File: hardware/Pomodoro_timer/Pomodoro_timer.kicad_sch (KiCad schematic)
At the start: 0 parts

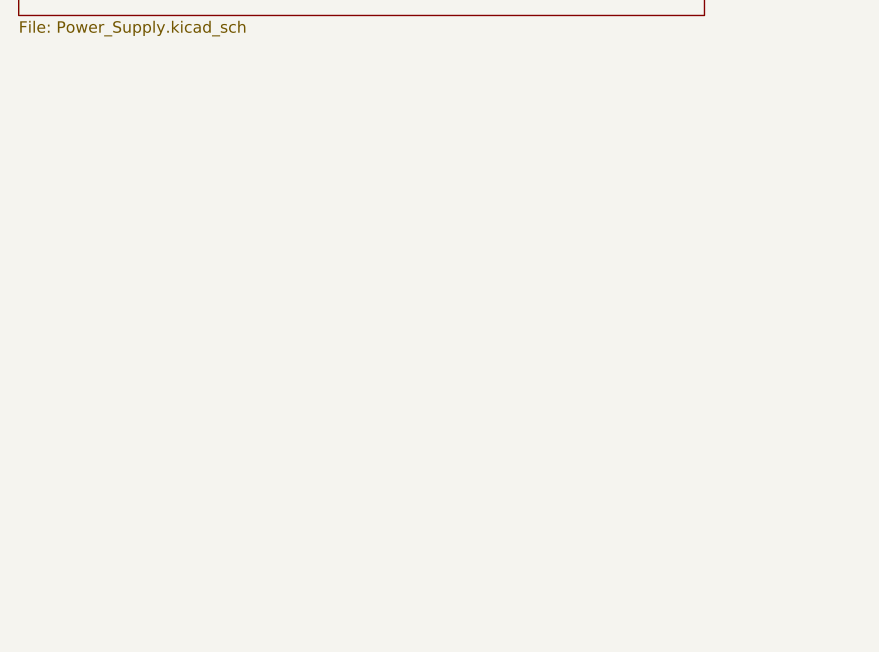
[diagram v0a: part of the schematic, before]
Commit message: PCB Ver.A : The Schematic completed the next part for PCB can be started.
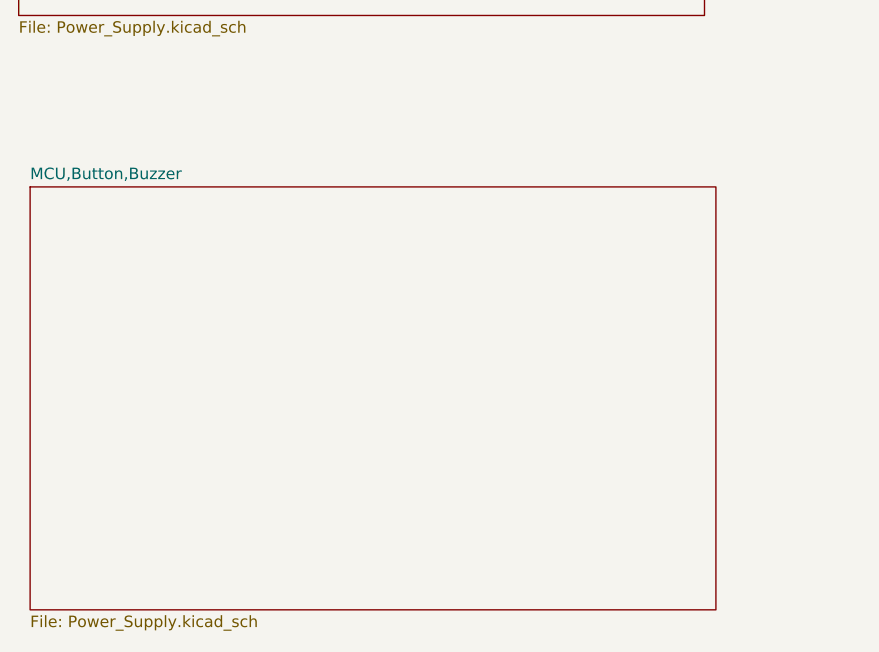
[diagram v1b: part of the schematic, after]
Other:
- added sheet MCU,Button,Buzzer (Power_Supply.kicad_sch)
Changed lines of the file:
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@@
+	)
+	(sheet
+		(at 17.78 82.55)
+		(size 76.2 46.99)
+		(exclude_from_sim no)
+		(in_bom yes)
+		(on_board yes)
+		(dnp no)
+		(fields_autoplaced yes)
+		(stroke
+			(width 0.1524)
+			(type solid)
+		)
+		(fill
+			(color 0 0 0 0.0000)
+		)
+		(property "Sheetname" "MCU,Button,Buzzer"
+			(at 17.78 81.8384 0)
+			(effects
+				(font
+					(size 1.27 1.27)
+				)
+				(justify left bottom)
+			)
+		)
+		(property "Sheetfile" "Power_Supply.kicad_sch"
+			(at 17.78 130.1246 0)
+			(effects
+				(font
+					(size 1.27 1.27)
+				)
+				(justify left top)
+			)
+		)
+		(instances
+			(project "Pomodoro_timer"
+				(path "/de804b87-618c-4b40-9e9d-dfdac3d4076a"
+					(page "4")
+				)
+			)
+		)
 	)
 	(sheet
